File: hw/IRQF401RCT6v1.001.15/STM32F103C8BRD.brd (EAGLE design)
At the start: 70 x 53.2 mm, 107 parts, among them IC2 LM1117IMPX-3.3, IC3 LM1117MPX-5.0, IC4 STM32F401RCT, P1 FSM, Q1 8MHz, Q2 32.768kHz, Q3 BC846BSMD, Q4 BSS84, Q5 MOSFET-PCH_SO-8, U1 24AA128-I/SN, U2 LTC1480CS8PBF

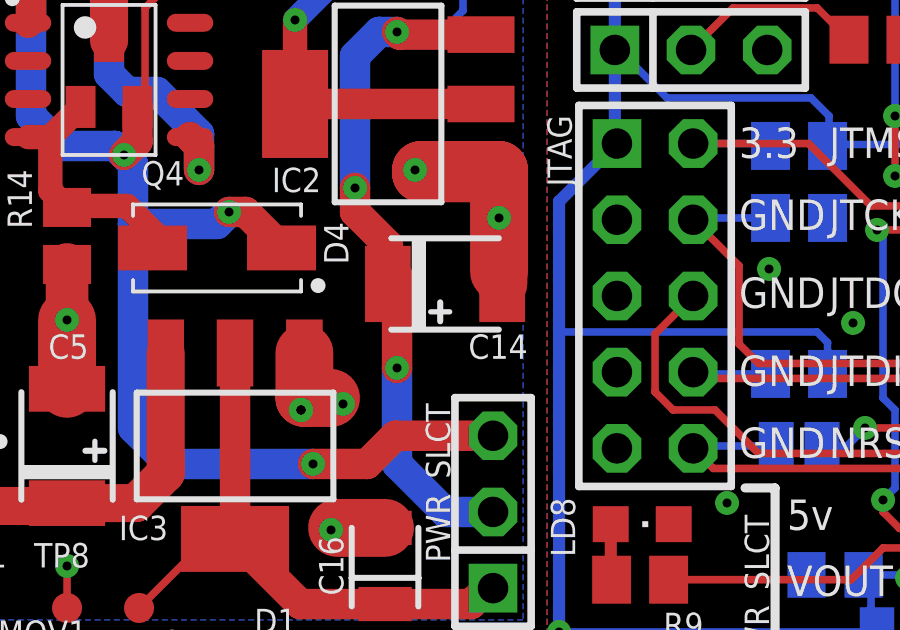
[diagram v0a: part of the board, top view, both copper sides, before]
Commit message: rev
New revision
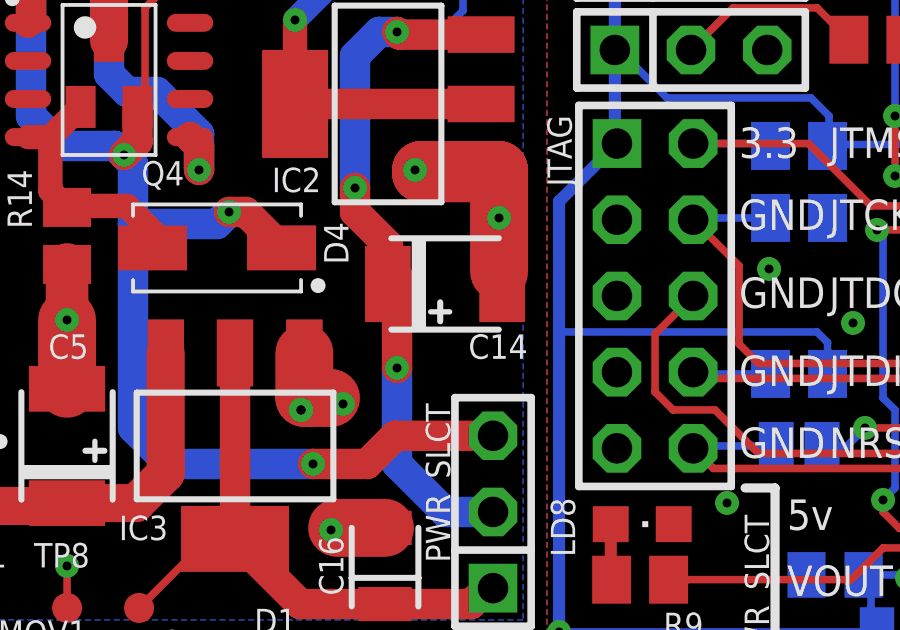
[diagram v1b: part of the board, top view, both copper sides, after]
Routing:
- net AGND: track 74.7 -> 73.9 mm
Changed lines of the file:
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@@
 <?xml version="1.0" encoding="utf-8"?>
 <!DOCTYPE eagle SYSTEM "eagle.dtd">
-<eagle version="7.6.0">
+<eagle version="9.0.0">
 <drawing>
 <settings>
-<setting alwaysvectorfont="no"/>
+<setting alwaysvectorfont="yes"/>
+<setting keepoldvectorfont="yes"/>
 <setting verticaltext="up"/>
 </settings>
@@
 <param name="dpMaxLengthDifference" value="10mm"/>
 <param name="dpGapFactor" value="2.5"/>
-<param name="checkGrid" value="0"/>
 <param name="checkAngle" value="1"/>
 <param name="checkFont" value="1"/>
 <param name="checkRestrict" value="1"/>
+<param name="checkStop" value="0"/>
+<param name="checkValues" value="0"/>
 <param name="useDiameter" value="13"/>
 <param name="maxErrors" value="50"/>
@@
 </element>
 <element name="X1" library="con-wago-500" package="W237-102" value="" x="4" y="36.8" smashed="yes" rot="R270">
+<attribute name="NAME" x="1.1962" y="37.6462" size="0.8128" layer="25" font="vector" ratio="15" rot="R270"/>
 <attribute name="VALUE" x="-3.62" y="41.84" size="1.27" layer="27" ratio="10" rot="R270"/>
-<attribute name="NAME" x="1.1962" y="37.6462" size="0.8128" layer="25" font="vector" ratio="15" rot="R270"/>
 </element>
 <element name="C19" library="cap-master" package="0805" value="20p" x="39.3" y="13.8" smashed="yes">
@@
 <element name="U2" library="LTC_By_element14_Batch_1" package="SOIC127P600X175-8N" value="LTC1480CS8PBF" x="28.3" y="5.4" smashed="yes" rot="R180">
 <attribute name="MPN" value="LTC1480CS8#PBF" x="28.3" y="5.4" size="1.778" layer="27" rot="R180" display="off"/>
+<attribute name="NAME" x="25.6456" y="1.845" size="0.8128" layer="25" font="vector" ratio="15" rot="SR0"/>
+<attribute name="OC_FARNELL" value="1663633" x="28.3" y="5.4" size="1.778" layer="27" rot="R180" display="off"/>
 <attribute name="OC_NEWARK" value="56M1547" x="28.3" y="5.4" size="1.778" layer="27" rot="R180" display="off"/>
+<attribute name="PACKAGE" value="SOIC-8" x="28.3" y="5.4" size="1.778" layer="27" rot="R180" display="off"/>
 <attribute name="SUPPLIER" value="Linear Technology" x="28.3" y="5.4" size="1.778" layer="27" rot="R180" display="off"/>
-<attribute name="PACKAGE" value="SOIC-8" x="28.3" y="5.4" size="1.778" layer="27" rot="R180" display="off"/>
-<attribute name="OC_FARNELL" value="1663633" x="28.3" y="5.4" size="1.778" layer="27" rot="R180" display="off"/>
-<attribute name="NAME" x="25.6456" y="1.845" size="0.8128" layer="25" font="vector" ratio="15" rot="SR0"/>
 <attribute name="VALUE" x="25.6456" y="0.885" size="0.8128" layer="27" font="vector" ratio="15" rot="SR0"/>
 </element>
@@
 <attribute name="DESCRIPTION" value="128K I2C CMOS Serial EEPROM" x="42.9" y="5.4" size="1.778" layer="27" display="off"/>
 <attribute name="MPN" value="24AA128-I/SN" x="42.9" y="5.4" size="1.778" layer="27" display="off"/>
+<attribute name="NAME" x="40.7788" y="1.8956" size="0.8128" layer="25" font="vector" ratio="15" rot="SR0"/>
+<attribute name="OC_FARNELL" value="-" x="42.9" y="5.4" size="1.778" layer="27" display="off"/>
 <attribute name="OC_NEWARK" value="92C6842" x="42.9" y="5.4" size="1.778" layer="27" display="off"/>
+<attribute name="PACKAGE" value="SOIC-8" x="42.9" y="5.4" size="1.778" layer="27" display="off"/>
 <attribute name="SUPPLIER" value="Microchip" x="42.9" y="5.4" size="1.778" layer="27" display="off"/>
-<attribute name="PACKAGE" value="SOIC-8" x="42.9" y="5.4" size="1.778" layer="27" display="off"/>
-<attribute name="OC_FARNELL" value="-" x="42.9" y="5.4" size="1.778" layer="27" display="off"/>
-<attribute name="NAME" x="40.7788" y="1.8956" size="0.8128" layer="25" font="vector" ratio="15" rot="SR0"/>
 <attribute name="VALUE" x="40.7374" y="0.8978" size="0.8128" layer="27" font="vector" ratio="15" rot="SR0"/>
 </element>
@@
 </element>
 <element name="X3" library="con-wago-500" package="W237-102" value="" x="4" y="17.8" smashed="yes" rot="R270">
+<attribute name="NAME" x="1.7962" y="18.6462" size="0.8128" layer="25" font="vector" ratio="15" rot="R270"/>
 <attribute name="VALUE" x="-3.62" y="22.84" size="1.27" layer="27" ratio="10" rot="R270"/>
-<attribute name="NAME" x="1.7962" y="18.6462" size="0.8128" layer="25" font="vector" ratio="15" rot="R270"/>
 </element>
 <element name="H5" library="holes" package="3,0-PAD" value="MOUNT-PAD-ROUND3.0" x="19.2" y="4"/>
@@
 </element>
 <element name="C5" library="cap-master" package="3528-TE-B" value="" x="10.4" y="28.2" smashed="yes" rot="R270">
+<attribute name="NAME" x="9.7775" y="31.105" size="0.8128" layer="25" font="vector" ratio="15"/>
 <attribute name="VALUE" x="7.5425" y="30.4225" size="0.8128" layer="27" ratio="14" rot="R270"/>
-<attribute name="NAME" x="9.7775" y="31.105" size="0.8128" layer="25" font="vector" ratio="15"/>
 </element>
 <element name="C14" library="cap-master" package="3528-TE-B" value="" x="23" y="33.6" smashed="yes" rot="R180">
+<attribute name="NAME" x="23.7775" y="31.105" size="0.8128" layer="25" font="vector" ratio="15"/>
 <attribute name="VALUE" x="25.2225" y="36.4575" size="0.8128" layer="27" ratio="14" rot="R180"/>
-<attribute name="NAME" x="23.7775" y="31.105" size="0.8128" layer="25" font="vector" ratio="15"/>
 </element>
 <element name="C16" library="cap-master" package="3216-TE-A" value="" x="21" y="24.2" smashed="yes" rot="R270">
+<attribute name="NAME" x="19.6125" y="23.2125" size="0.8128" layer="25" font="vector" ratio="15" rot="R90"/>
 <attribute name="VALUE" x="18.7775" y="25.7875" size="0.8128" layer="27" ratio="14" rot="R270"/>
-<attribute name="NAME" x="19.6125" y="23.2125" size="0.8128" layer="25" font="vector" ratio="15" rot="R90"/>
 </element>
 <element name="C17" library="cap-master" package="3216-TE-A" value="" x="23.2" y="44.6" smashed="yes" rot="R180">
+<attribute name="NAME" x="21.8125" y="45.9875" size="0.8128" layer="25" font="vector" ratio="15"/>
 <attribute name="VALUE" x="24.7875" y="46.8225" size="0.8128" layer="27" ratio="14" rot="R180"/>
-<attribute name="NAME" x="21.8125" y="45.9875" size="0.8128" layer="25" font="vector" ratio="15"/>
 </element>
 <element name="J1" library="con-jack" package="SPC4078" value="" x="5.4" y="48.2" smashed="yes">
+<attribute name="NAME" x="5.04" y="51.08" size="0.8128" layer="25" font="vector" ratio="15"/>
 <attribute name="VALUE" x="-4.76" y="41.85" size="1.27" layer="27"/>
-<attribute name="NAME" x="5.04" y="51.08" size="0.8128" layer="25" font="vector" ratio="15"/>
 </element>
 <element name="L4" library="ipc-7351-inductor" package="INDC1608X95N" value="10uH" x="6.2" y="26.2" smashed="yes">
@@
 <element name="C9" library="ipc-7351-capacitor" package="CAPC3215X168N" value="" x="29" y="49.6" rot="MR90"/>
 <element name="X2" library="con-wago-500" package="W237-102" value="" x="4" y="6.8" smashed="yes" rot="R270">
+<attribute name="NAME" x="1.7962" y="7.4462" size="0.8128" layer="25" font="vector" ratio="15" rot="R270"/>
 <attribute name="VALUE" x="-3.62" y="11.84" size="1.27" layer="27" ratio="10" rot="R270"/>
-<attribute name="NAME" x="1.7962" y="7.4462" size="0.8128" layer="25" font="vector" ratio="15" rot="R270"/>
 </element>
 <element name="MOV1" library="varistor" package="VARC2012X70N" value="" x="9.2" y="20" smashed="yes" rot="R90">
@@
 <wire x1="10.4" y1="30.105" x2="10.4" y2="32.4" width="1.9304" layer="1"/>
 <wire x1="10.4" y1="34.25" x2="10.4" y2="32.4" width="1.4224" layer="1"/>
-<wire x1="24.905" y1="33.6" x2="24.8" y2="34.305" width="1.016" layer="1"/>
 <wire x1="42.9" y1="47.95" x2="42.8" y2="48.05" width="0.254" layer="16"/>
 <wire x1="42.8" y1="48.05" x2="42.8" y2="49" width="0.254" layer="16"/>
@@
 <wire x1="10.4" y1="24.2" x2="10.6" y2="24.2" width="0.254" layer="16"/>
 <contactref element="C8" pad="2"/>
-<wire x1="24.905" y1="33.6" x2="24.905" y2="34" width="1.6764" layer="1"/>
-<wire x1="24.905" y1="34" x2="24.8" y2="34" width="1.6764" layer="1"/>
 <wire x1="24.8" y1="34" x2="24.8" y2="37.4" width="1.9304" layer="1"/>
 <wire x1="24.8" y1="37.4" x2="22.2" y2="37.4" width="1.9304" layer="1"/>
@@
 <via x="15.2" y="51.8" extent="1-16" drill="0.3"/>
 <wire x1="11.436" y1="51.746" x2="13.584" y2="51.746" width="1.27" layer="1"/>
+<wire x1="24.905" y1="33.6" x2="24.905" y2="33.895" width="0.1524" layer="1"/>
+<wire x1="24.905" y1="33.895" x2="24.8" y2="34" width="0.1524" layer="1"/>
 <wire x1="22" y1="37.4" x2="22.2" y2="37.4" width="0" layer="19" extent="1-1"/>
 </signal>
@@
 <wire x1="21.4" y1="27.6" x2="21.4" y2="30.8" width="1.016" layer="16"/>
 <via x="21.4" y="30.8" extent="1-16" drill="0.3"/>
-<wire x1="21.4" y1="30.8" x2="21.4" y2="33.895" width="1.016" layer="1"/>
-<wire x1="21.4" y1="33.895" x2="21.095" y2="33.6" width="1.016" layer="1"/>
+<wire x1="21.4" y1="33.895" x2="21.4" y2="30.8" width="1.016" layer="1"/>
 <wire x1="23.6" y1="42.711" x2="22.8" y2="41.911" width="0.254" layer="16"/>
 <wire x1="22.8" y1="41.911" x2="21.489" y2="41.911" width="0.254" layer="16"/>
@@
 <contactref element="PWR_SLCT" pad="2"/>
 <wire x1="23" y1="26" x2="24.6" y2="26" width="1.016" layer="16"/>
+<wire x1="21.095" y1="33.6" x2="21.105" y2="33.6" width="0.1524" layer="1"/>
+<wire x1="21.105" y1="33.6" x2="21.4" y2="33.895" width="0.1524" layer="1"/>
 </signal>
 <signal name="VSSA">
